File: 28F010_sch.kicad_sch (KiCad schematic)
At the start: 12 parts, among them U10 74LVC1G332, U11 74LS138, U12 CY7C199, U15 CY7C199, U16 4012, U17 CY7C199, U8 74LS138, U9 CY7C199

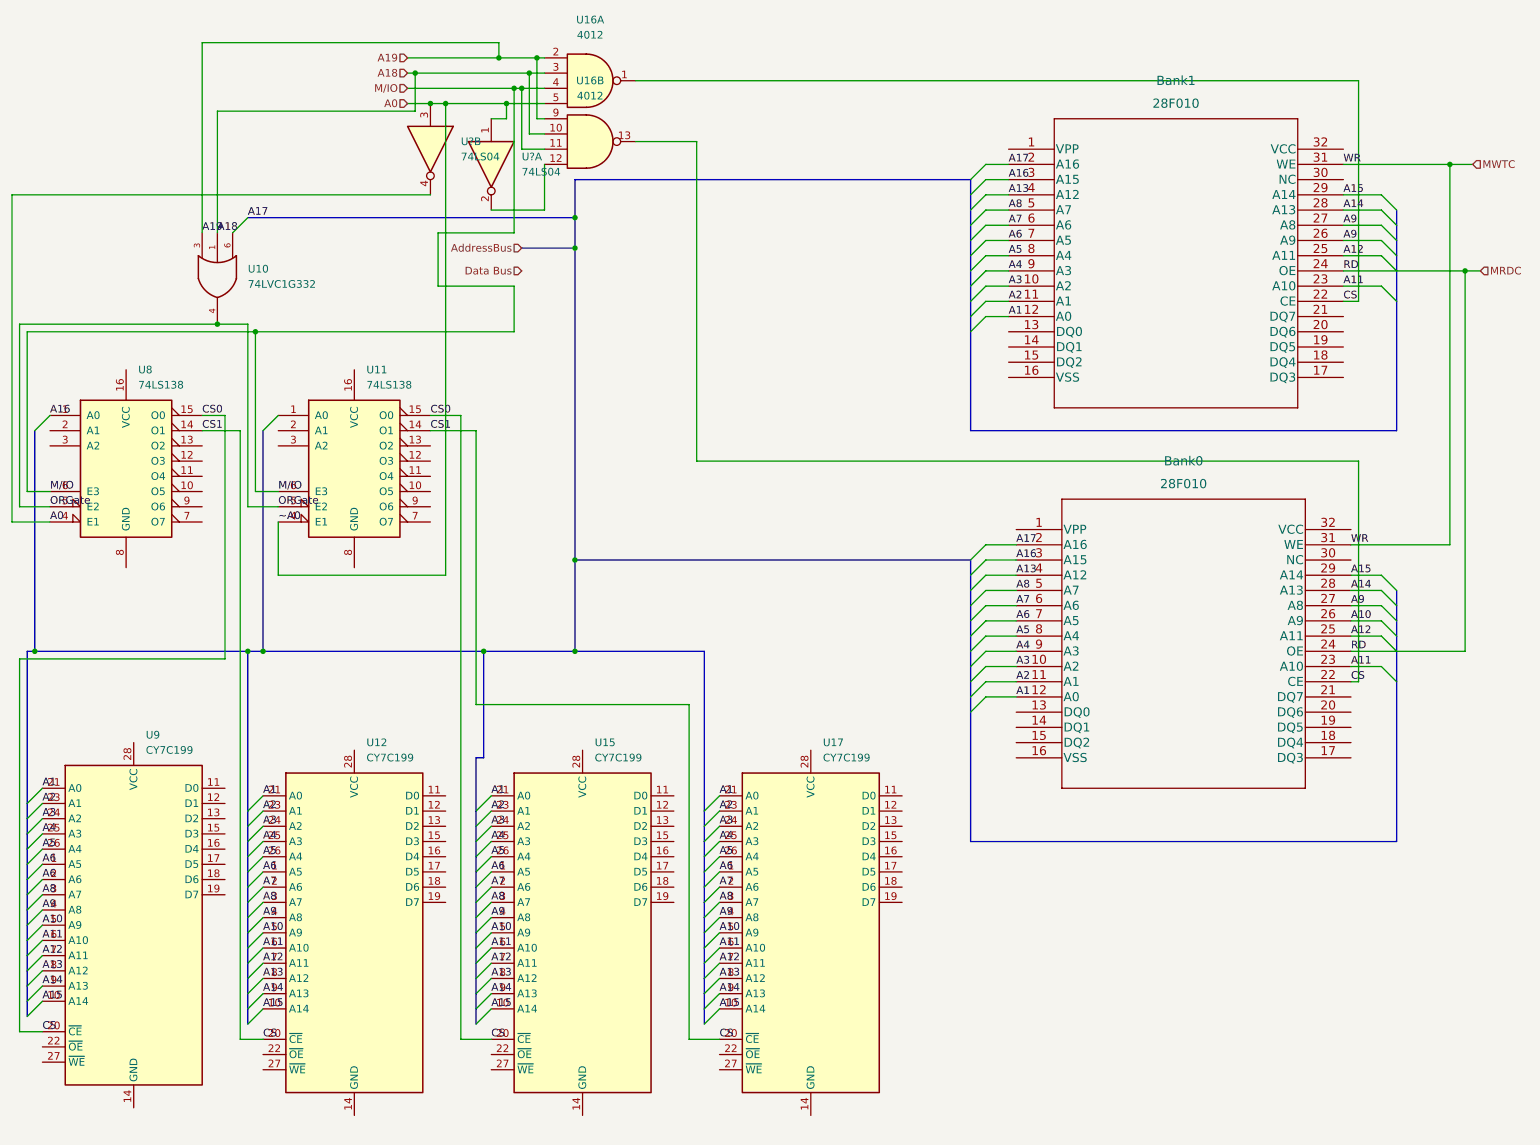
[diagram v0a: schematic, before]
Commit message: Added the databus
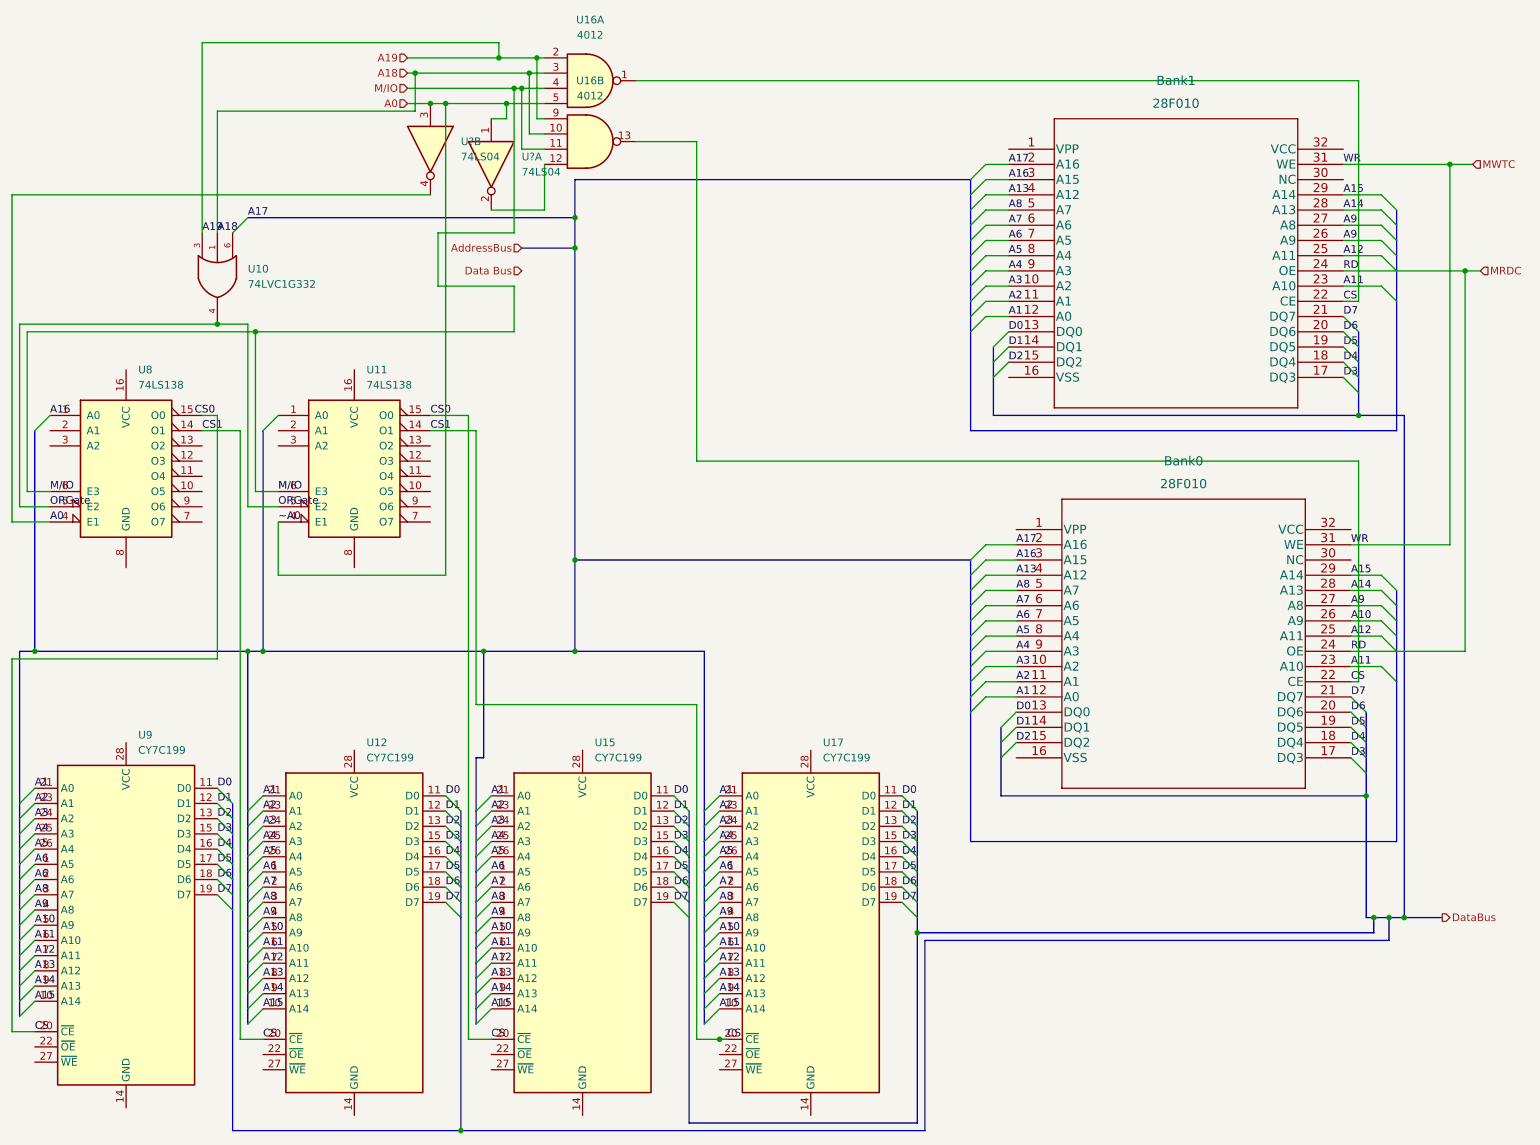
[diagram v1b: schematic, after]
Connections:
- net D0: now reaches Bank0.13 (DQ0)
- net D0: now also Bank1.13 (DQ0), U12.11 (D0), U15.11 (D0), U17.11 (D0), U9.11 (D0)
- net D1: now reaches Bank0.14 (DQ1)
- net D1: now also Bank1.14 (DQ1), U12.12 (D1), U15.12 (D1), U17.12 (D1), U9.12 (D1)
- net D2: now reaches Bank0.15 (DQ2)
- net D2: now also Bank1.15 (DQ2), U12.13 (D2), U15.13 (D2), U17.13 (D2), U9.13 (D2)
- net D3: now reaches Bank0.17 (DQ3)
- net D3: now also Bank1.17 (DQ3), U12.15 (D3), U15.15 (D3), U17.15 (D3), U9.15 (D3)
- net D4: now reaches Bank0.18 (DQ4)
- net D4: now also Bank1.18 (DQ4), U12.16 (D4), U15.16 (D4), U17.16 (D4), U9.16 (D4)
- net D5: now reaches Bank0.19 (DQ5)
- net D5: now also Bank1.19 (DQ5), U12.17 (D5), U15.17 (D5), U17.17 (D5), U9.17 (D5)
- net D6: now reaches Bank0.20 (DQ6)
- net D6: now also Bank1.20 (DQ6), U12.18 (D6), U15.18 (D6), U17.18 (D6), U9.18 (D6)
- net D7: now reaches Bank0.21 (DQ7)
- net D7: now also Bank1.21 (DQ7), U12.19 (D7), U15.19 (D7), U17.19 (D7), U9.19 (D7)
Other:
- moved on the sheet: U9
